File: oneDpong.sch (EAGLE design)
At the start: 70 parts, among them IC1 MEGA8-AI, IC2 74HC257D, IC3 LM386M-1, IC4 NPIC6C596, IC5 NPIC6C596, Q2 NTD5867NL_NMOSFET, Q3 SCR_BT300S

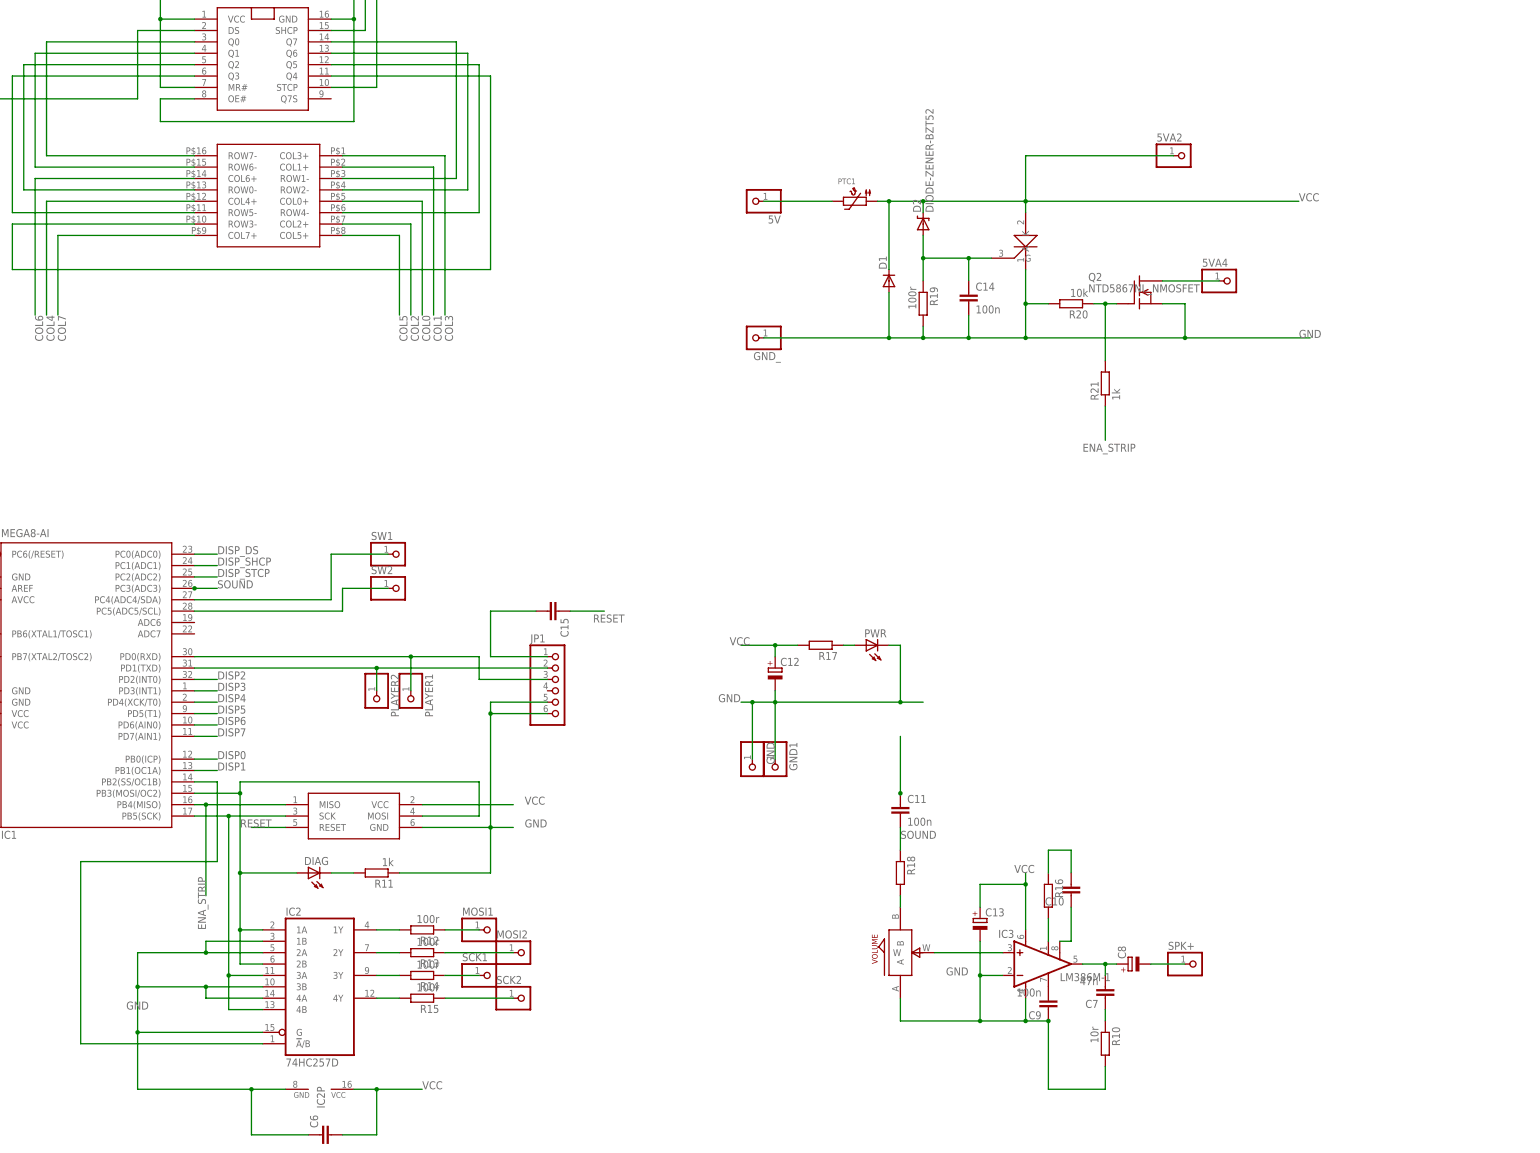
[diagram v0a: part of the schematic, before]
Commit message: poss V3
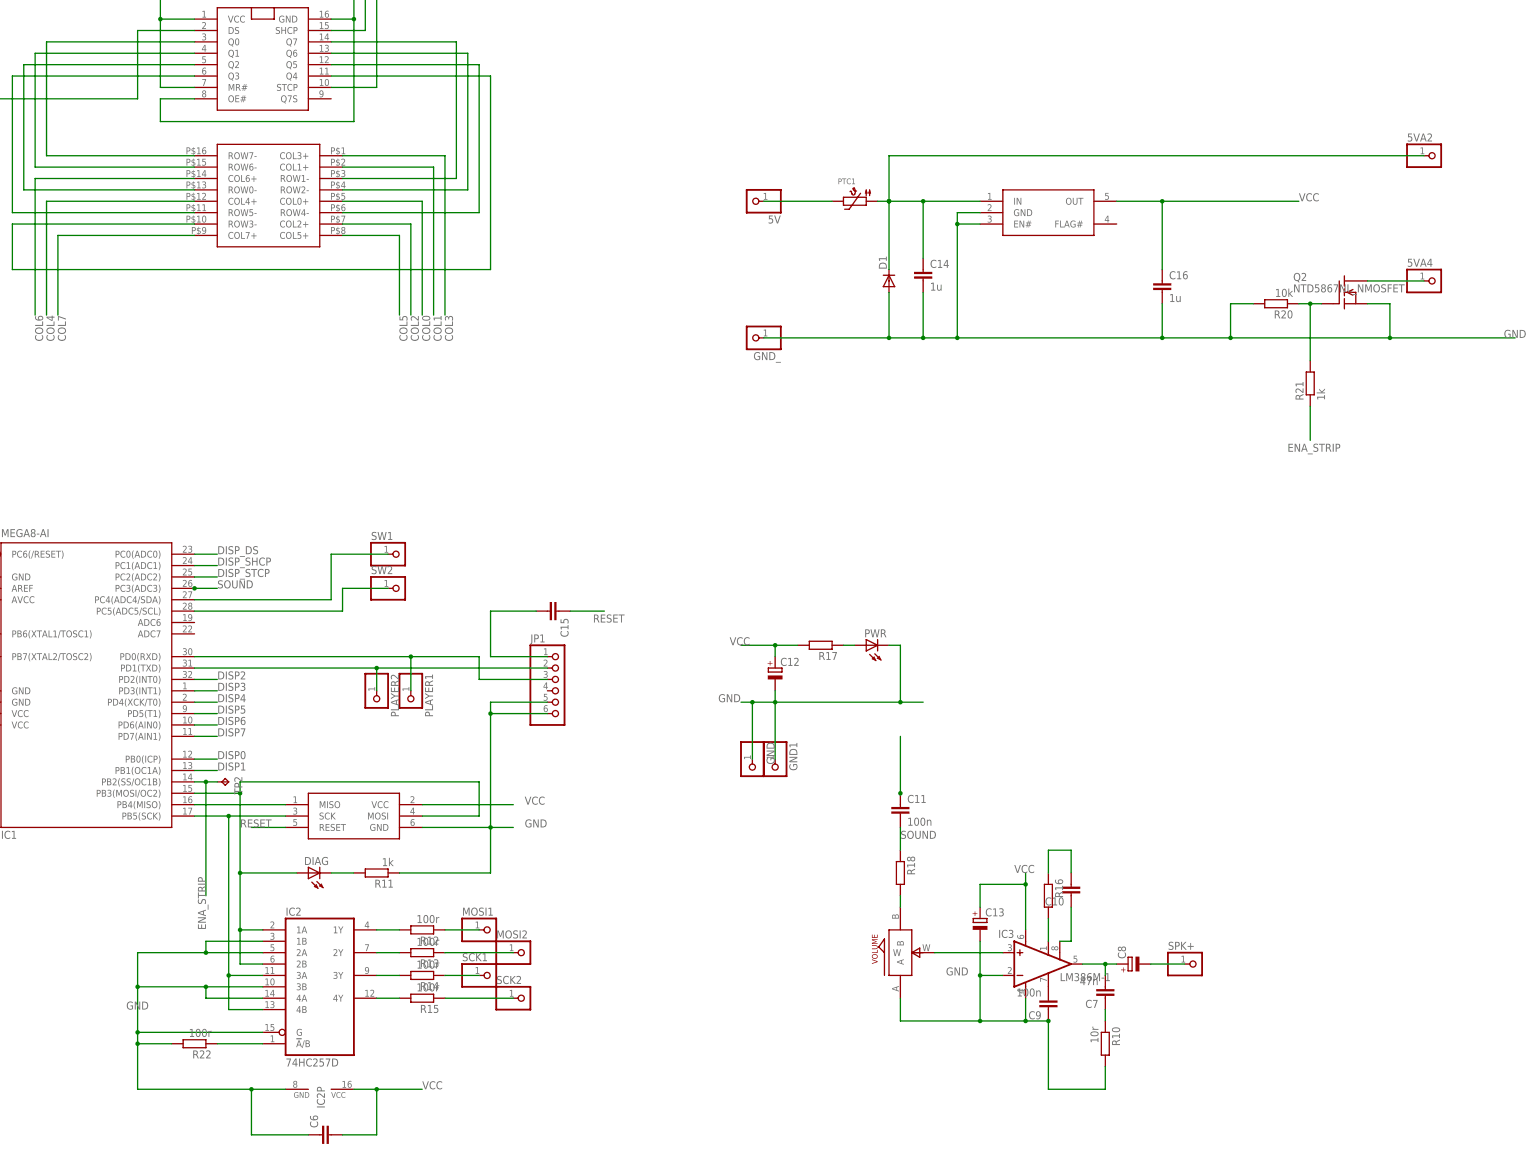
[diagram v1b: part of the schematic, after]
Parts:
- removed D2: DIODE-ZENER-BZT52, SparkFun:DIODE-ZENER-BZT52
- removed Q3: SCR_BT300S, jason_eagle6:SCR_BT300S
- removed R19: 100r, rcl:R-EU_R0805
- added C16: 1u, rcl:C-EUC0805
- added IC6: NCP361SNT1G, jason_eagle6:NCP361SNT1G
- added R22: 100r, rcl:R-EU_R0805
- added TP2: TPB2,54, testpad:TPB2,54
- C14: value 100n -> 1u
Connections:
- removed net N$13: IC1.PB2(SS/OC1B), IC2A.!A!/B
- removed net N$31: C14.1, D2.A, Q3.G, R19.1
- new net MISO: IC1.PB4(MISO), ICSP.MISO
- new net N$2: IC2A.!A!/B, R22.1
- new net VIN: 5VA2.1, C14.1, D1.C, IC6.IN, PTC1.1
- net ENA_STRIP: now also IC1.PB2(SS/OC1B), TP2.TP; no longer IC1.PB4(MISO), ICSP.MISO
- net GND: now also C16.2, IC6.EN#, IC6.GND, R22.2; no longer Q3.K, R19.2
- net VCC: now also C16.1, IC6.OUT; no longer 5VA2.1, D1.C, D2.C, PTC1.1, Q3.A
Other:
- moved on the sheet: 5VA2, 5VA4, C14, Q2, R20, R21

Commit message: V3 BOARD
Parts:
- removed R22: 100r, rcl:R-EU_R0805
- removed TP2: TPB2,54, testpad:TPB2,54
- added R19: 1k, rcl:R-EU_R0805
- added TP1: TPB1,27, testpad:TPB1,27
- added X1: (no value), crystal:CRYSTALHC49U-V
- C10: value (none) -> 47n
- C11: value 100n -> (none)
- C12, C13: value (none) -> 100n; device rcl:CPOL-EUE2.5-6 -> rcl:C-EUC0805
- C14: value 1u -> (none)
- C15: value (none) -> 1u
- C4: device rcl:C-EUC0805 -> rcl:CPOL-EUE2.5-6
- C7: value 47n -> (none)
- C9: value 100n -> (none); device rcl:C-EUC0805 -> rcl:CPOL-EUE2.5-6
- IC1: value MEGA8-AI -> NPIC6C596; device atmel:MEGA8-AI -> jasons_stuff:NPIC6C596
- IC3: value LM386M-1 -> MEGA8-AI; device linear:LM386M-1 -> atmel:MEGA8-AI
- IC4: value NPIC6C596 -> LM386M-1; device jasons_stuff:NPIC6C596 -> linear:LM386M-1
- Q1: value (none) -> SPD30P06PTO252; device crystal:CRYSTALHC49U-V -> transistor-fet:SPD30P06PTO252
- Q2: value NTD5867NL_NMOSFET -> (none); device jason_eagle6:NTD5867NL_NMOSFET -> transistor:MMBT3904LT1-NPN-SOT23-BEC
- R10: value 10r -> 100r
- R11: value 1k -> 100r
- R13: value 100r -> 10r
- R14, R15, R7: value 100r -> (none)
- R16, R17, R18, R9: value (none) -> 100r
- R21: value 1k -> (none)
- R6: value 100r -> 1k
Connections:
- removed net N$32: 5VA4.1, Q2.D
- removed net Z: Q2.G, R20.1, R21.2
- new net N$13: 5VA2.1, Q1.D
- new net N$29: Q1.G, Q2.C, R20.2
- new net N$30: Q2.B, R19.1
- net COL0: now also R9.2; no longer R6.2
- net COL1: now also R8.2; no longer R7.2
- net COL2: now also R18.2; no longer R5.2
- net COL3: now also R17.2; no longer R8.2
- net COL4: now also R16.2; no longer R2.2
- net COL5: now also R12.2; no longer R4.2
- net COL6: now also R10.2; no longer R1.2
- net COL7: now also R11.2; no longer R3.2
- net DISP0: now also IC3.PB0(ICP), R9.1; no longer IC1.PB0(ICP), R6.1
- net DISP1: now also IC3.PB1(OC1A), R8.1; no longer IC1.PB1(OC1A), R7.1
- net DISP2: now also IC3.PD2(INT0), R18.1; no longer IC1.PD2(INT0), R5.1
- net DISP3: now also IC3.PD3(INT1), R17.1; no longer IC1.PD3(INT1), R8.1
- net DISP4: now also IC3.PD4(XCK/T0), R16.1; no longer IC1.PD4(XCK/T0), R2.1
- net DISP5: now also IC3.PD5(T1), R12.1; no longer IC1.PD5(T1), R4.1
- net DISP6: now also IC3.PD6(AIN0), R10.1; no longer IC1.PD6(AIN0), R1.1
- net DISP7: now also IC3.PD7(AIN1), R11.1; no longer IC1.PD7(AIN1), R3.1
- net DISP_DS: now also IC3.PC0(ADC0); no longer IC1.PC0(ADC0)
- net DISP_DS2: now also IC1.DS; no longer IC4.DS
- net DISP_SHCP: now also IC1.SHCP, IC3.PC1(ADC1); no longer IC1.PC1(ADC1), IC4.SHCP
- net DISP_STCP: now also IC1.STCP, IC3.PC2(ADC2); no longer IC1.PC2(ADC2), IC4.STCP
- net ENA_STRIP: now also IC3.PB2(SS/OC1B), R19.2, TP1.TP; no longer IC1.PB2(SS/OC1B), R21.1, TP2.TP
- net GND: now also 5VA4.1, C12.1, C15.2, C4.-, C7.1, C9.-, IC1.OE#, IC3.GND@1, IC3.GND@2, IC4.-IN, Q2.E, R1.2, R13.2, R6.1; no longer C1.2, C12.-, C13.-, C4.1, C9.1, IC1.GND@1, IC1.GND@2, IC3.-IN, IC4.OE#, Q2.S, R10.2, R11.1, R20.2, R22.2
- net MISO: now also IC3.PB4(MISO); no longer IC1.PB4(MISO)
- net MOSI2: now also R4.1; no longer R13.1
- net N$1: now also IC3.PD0(RXD); no longer IC1.PD0(RXD)
- net N$10: now also R3.2; no longer R14.2
- net N$11: now also R5.2; no longer R15.2
- net N$12: now also R2.1; no longer R12.1
- net N$14: now also IC3.PD1(TXD); no longer IC1.PD1(TXD)
- net N$15: now also R5.1; no longer R15.1
- net N$16: now also R14.2; no longer R18.2
- net N$17: now also IC4.+IN; no longer IC3.+IN
- net N$18: now also IC3.PC5(ADC5/SCL); no longer IC1.PC5(ADC5/SCL)
- net N$19: now also C10.2, IC4.OUT; no longer C7.2, IC3.OUT
- net N$2: now also R1.1; no longer R22.1
- net N$21: now also C12.2, IC4.BYPASS; no longer C9.2, IC3.BYPASS
- net N$22: now also IC4.GAIN@1, R15.2; no longer IC3.GAIN@1, R16.2
- net N$23: now also C11.2, R15.1; no longer C10.2, R16.1
- net N$24: now also C11.1, IC4.GAIN@2; no longer C10.1, IC3.GAIN@2
- net N$25: now also C13.2, R14.1; no longer C11.2, R18.1
- net N$26: now also R21.1; no longer R17.1
- net N$27: now also R6.2; no longer R11.2
- net N$3: now also C7.2, IC3.PB6(XTAL1/TOSC1), X1.2; no longer C3.2, IC1.PB6(XTAL1/TOSC1), Q1.2
- net N$4: now also C6.2, IC3.PB7(XTAL2/TOSC2), X1.1; no longer C4.2, IC1.PB7(XTAL2/TOSC2), Q1.1
- net N$5: now also R2.2; no longer R12.2
- net N$6: now also R4.2; no longer R13.2
- net N$7: now also IC3.PB5(SCK); no longer IC1.PB5(SCK)
- net N$8: now also C10.1, R13.1; no longer C7.1, R10.1
- net N$9: now also C1.2; no longer C15.2
- net PMOSI: now also IC3.PB3(MOSI/OC2); no longer IC1.PB3(MOSI/OC2)
- net Q0A1: now also IC1.Q0; no longer IC4.Q0
- net Q1A1: now also IC1.Q1; no longer IC4.Q1
- net Q2A1: now also IC1.Q2; no longer IC4.Q2
- net Q3A1: now also IC1.Q3; no longer IC4.Q3
- net Q4A1: now also IC1.Q4; no longer IC4.Q4
- net Q5A1: now also IC1.Q5; no longer IC4.Q5
- net Q6A1: now also IC1.Q6; no longer IC4.Q6
- net Q7A1: now also IC1.Q7; no longer IC4.Q7
- net RESET: now also C1.1, IC3.PC6(/RESET), R7.1; no longer C15.1, IC1.PC6(/RESET), R9.1
- net SCK1: now also R3.1; no longer R14.1
- net SOUND: now also C13.1, IC3.PC3(ADC3); no longer C11.1, IC1.PC3(ADC3)
- net SW1: now also IC3.PC4(ADC4/SDA); no longer IC1.PC4(ADC4/SDA)
- net VCC: now also C14.1, C15.1, C3.2, C4.+, C9.+, IC1.MR#, IC1.VCC, IC3.AREF, IC3.AVCC, IC3.VCC@1, IC3.VCC@2, IC4.VS, R21.2, R7.2; no longer C1.1, C12.+, C13.+, C16.1, C6.2, IC1.AREF, IC1.AVCC, IC1.VCC@1, IC1.VCC@2, IC3.VS, IC4.MR#, IC4.VCC, R17.2, R9.2
- net VIN: now also C16.1, Q1.S, R20.1; no longer 5VA2.1, C14.1
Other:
- moved on the sheet: 5VA2, C1, C10, C11, C14, C15, C16, C3, C6, C7, Q2, R1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
